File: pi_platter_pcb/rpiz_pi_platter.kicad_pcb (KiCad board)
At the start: 2 copper layers, 65 x 30 mm, 7 parts, among them J1 GPIO_CONNECTOR, J2 BME680_CONNECTOR, J3 RFM95W_CONNECTOR

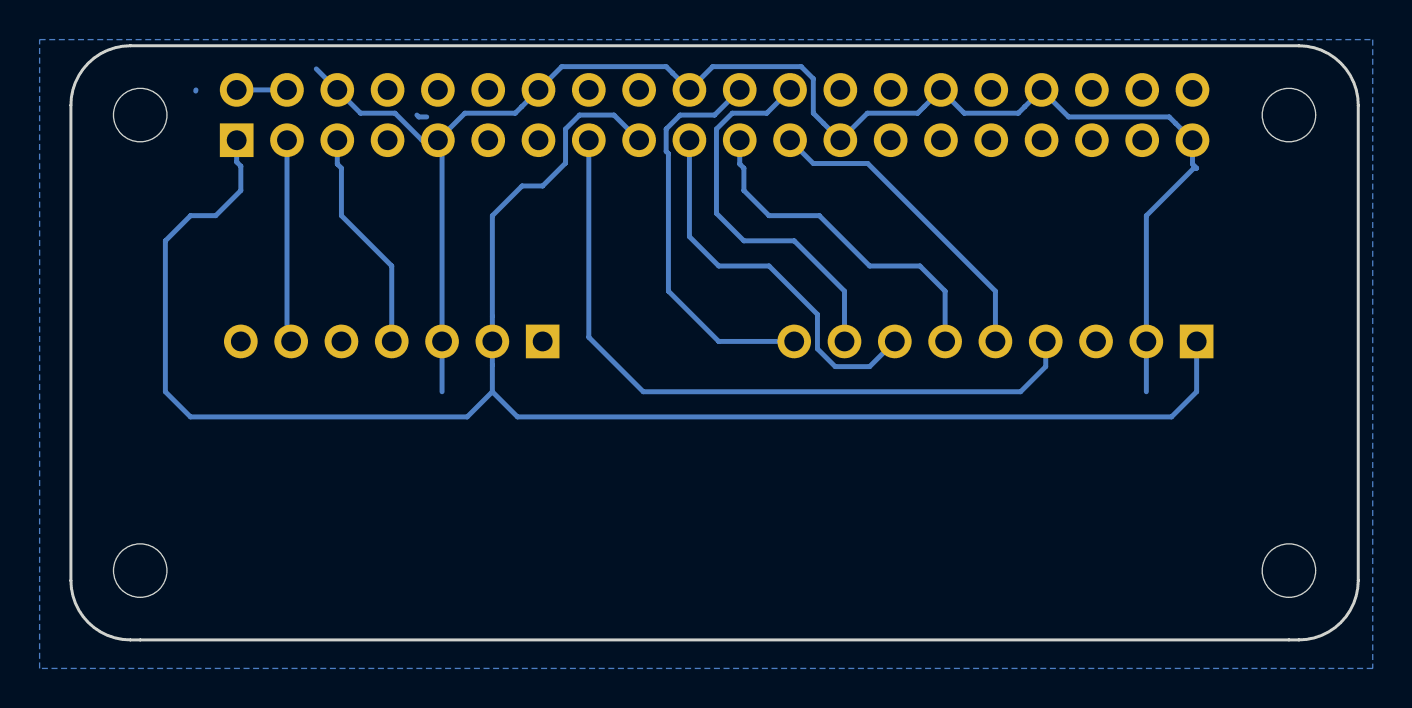
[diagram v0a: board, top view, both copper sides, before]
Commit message: modification of pcb
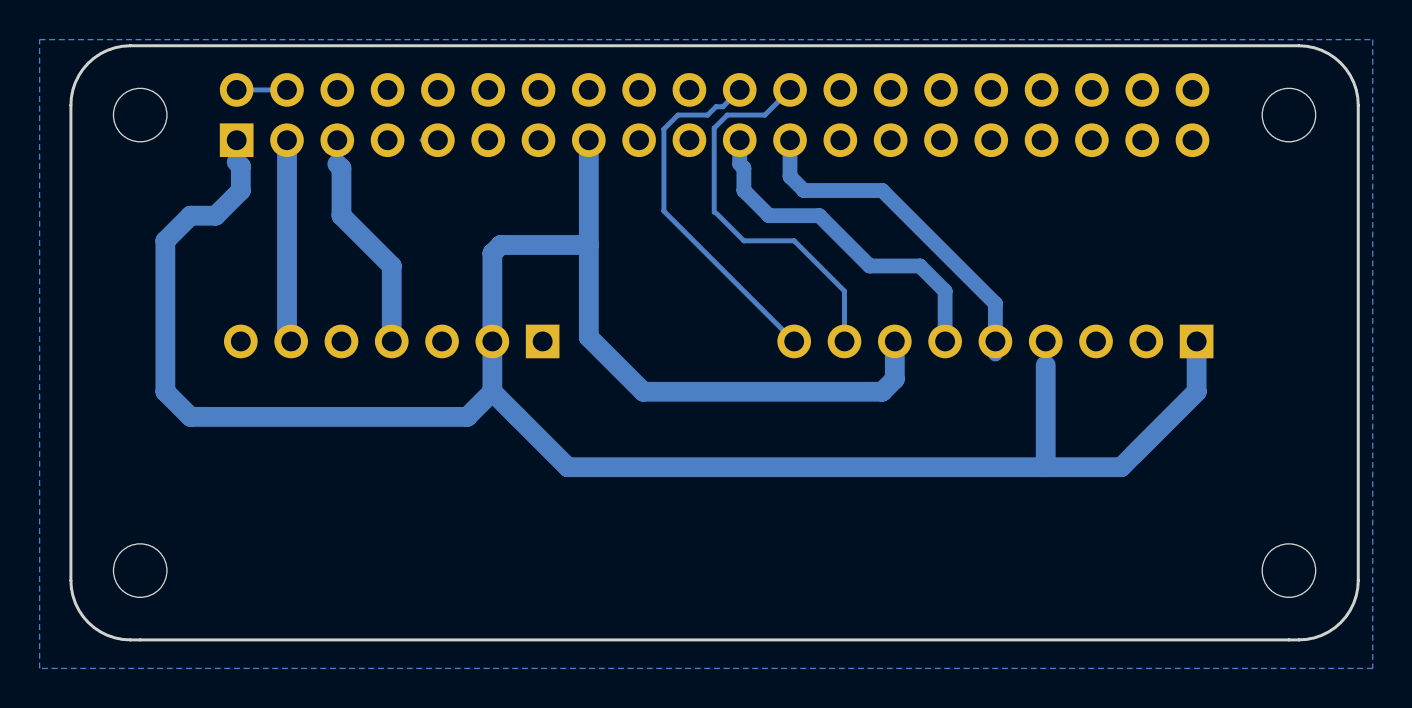
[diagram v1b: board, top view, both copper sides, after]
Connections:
- J1 pad 15: /GPIO22_GEN3 -> +3V3
- J1 pad 19: /GPIO10_SPI_MOSI -> +3V3
- J3 pad 4: /GPIO22_GEN3 -> +3V3
- J3 pad 7: /GPIO10_SPI_MOSI -> +3V3
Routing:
- net GND: track 80.6 -> 1.10 mm
- net /GPIO22_GEN3: track 36.0 -> 0.00 mm
- net +3V3: track 91.8 -> 125.5 mm
- net /GPIO10_SPI_MOSI: track 19.5 -> 0.00 mm
- net /GPIO25_GEN6: track 20.2 -> 18.1 mm
- net /GPIO11_SPI_SCLK: track 16.1 -> 17.4 mm
- net (no net): track 0.54 -> 0.00 mm
- added copper zone on B.Cu, net GND
- removed copper zone on B.Cu, net (none)
